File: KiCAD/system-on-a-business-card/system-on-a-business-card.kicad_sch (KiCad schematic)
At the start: 15 parts, among them J1 USB_C_Receptacle, J3 Conn_01x04_Socket, SW1 SW_Push, U1 USBLC6-2SC6

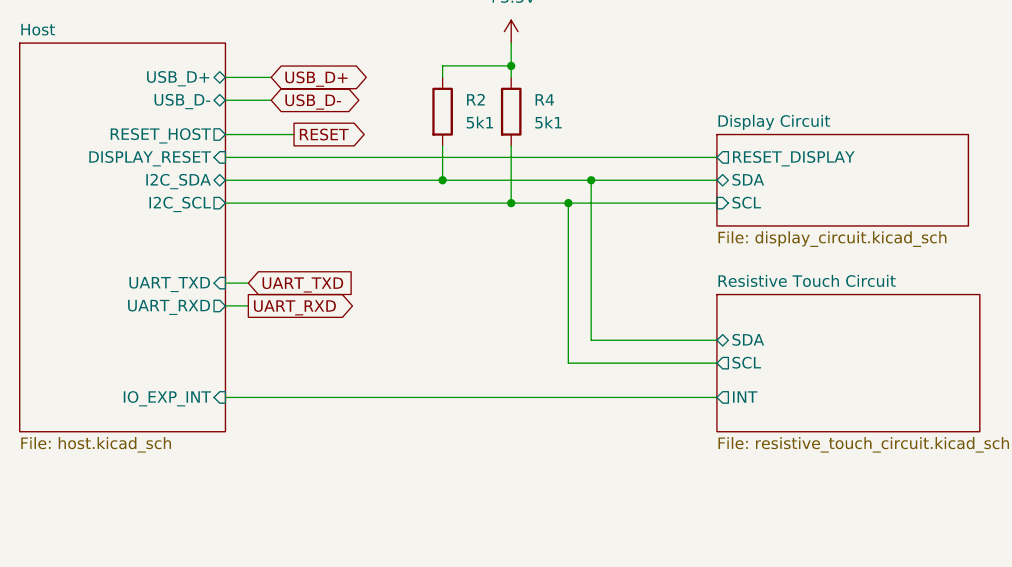
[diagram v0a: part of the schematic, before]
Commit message: #10: finished initial routing
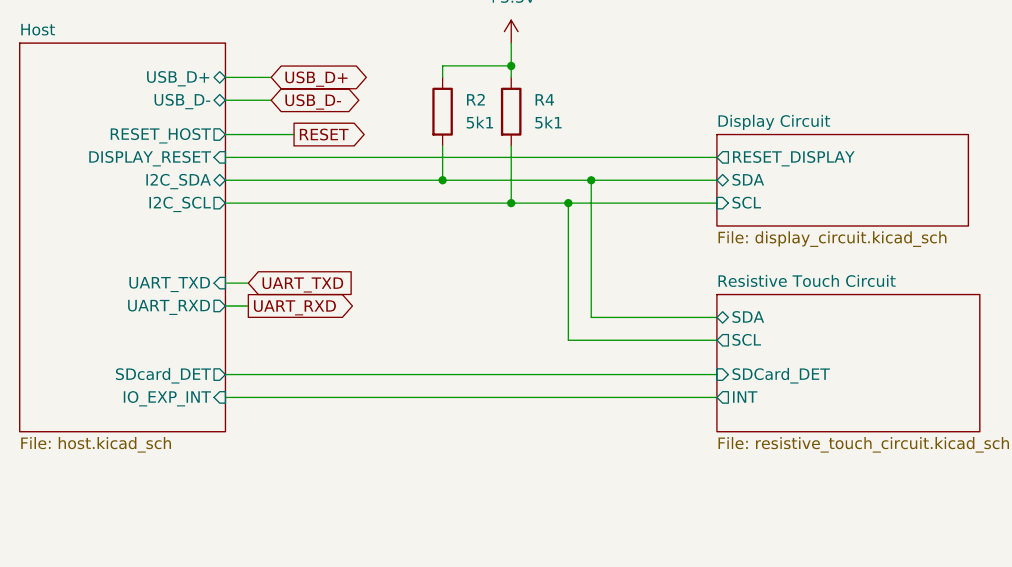
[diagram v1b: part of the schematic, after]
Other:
- sheet Host ports: added SDcard_DET; removed none
- sheet Resistive Touch Circuit ports: added SDCard_DET; removed none
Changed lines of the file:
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@@
     (stroke (width 0) (type default))
   )
-  (wire (pts (xy 102.87 67.31) (xy 102.87 49.53))
+  (wire (pts (xy 102.87 64.77) (xy 102.87 49.53))
     (stroke (width 0) (type default))
   )
@@
     (stroke (width 0) (type default))
   )
-  (wire (pts (xy 105.41 64.77) (xy 105.41 46.99))
+  (wire (pts (xy 105.41 62.23) (xy 105.41 46.99))
     (stroke (width 0) (type default))
   )
@@
     (stroke (width 0) (type default))
   )
-  (wire (pts (xy 119.38 64.77) (xy 105.41 64.77))
+  (wire (pts (xy 119.38 62.23) (xy 105.41 62.23))
     (stroke (width 0) (type default))
   )
@@
     (stroke (width 0) (type default))
   )
-  (wire (pts (xy 119.38 67.31) (xy 102.87 67.31))
+  (wire (pts (xy 119.38 64.77) (xy 102.87 64.77))
     (stroke (width 0) (type default))
   )
   (wire (pts (xy 64.77 35.56) (xy 69.85 35.56))
+    (stroke (width 0) (type default))
+  )
+  (wire (pts (xy 64.77 68.58) (xy 119.38 68.58))
     (stroke (width 0) (type default))
   )
@@
       (effects (font (size 1.27 1.27)) (justify left top))
     )
-    (pin "SDA" bidirectional (at 119.38 64.77 180)
-      (effects (font (size 1.27 1.27)) (justify left))
-    )
-    (pin "SCL" output (at 119.38 67.31 180)
+    (pin "SDA" bidirectional (at 119.38 62.23 180)
+      (effects (font (size 1.27 1.27)) (justify left))
+    )
+    (pin "SCL" output (at 119.38 64.77 180)
       (effects (font (size 1.27 1.27)) (justify left))
     )
     (pin "INT" output (at 119.38 71.12 180)
+      (effects (font (size 1.27 1.27)) (justify left))
+    )
+    (pin "SDCard_DET" input (at 119.38 68.58 180)
       (effects (font (size 1.27 1.27)) (justify left))
     )
@@
       (effects (font (size 1.27 1.27)) (justify right))
     )
+    (pin "SDcard_DET" output (at 64.77 68.58 0)
+      (effects (font (size 1.27 1.27)) (justify right))
+    )
